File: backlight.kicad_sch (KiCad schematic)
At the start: 32 parts

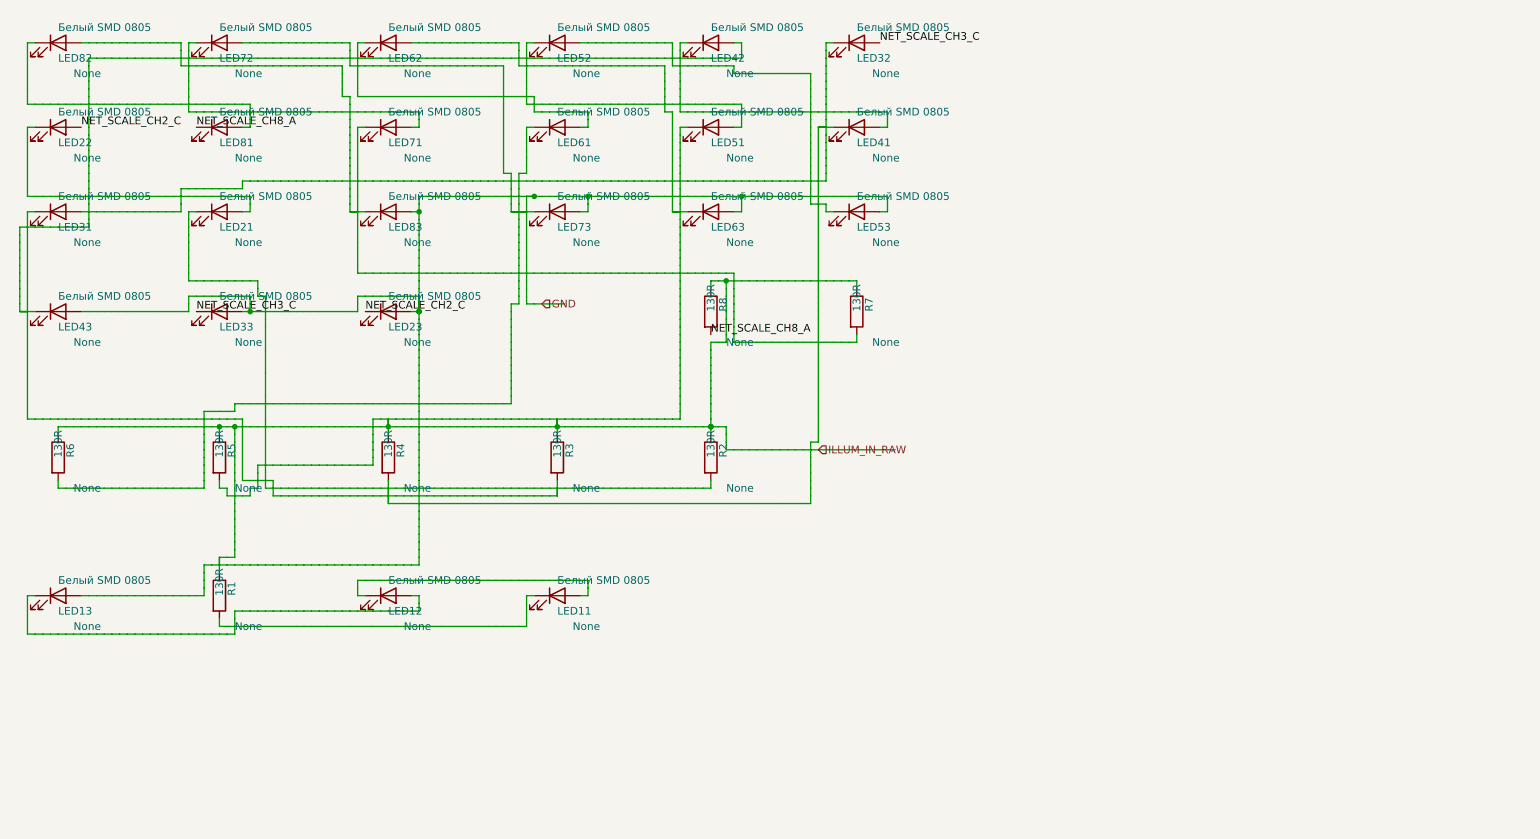
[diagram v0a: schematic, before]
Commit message: рефакторинг проекта и начала прогона тестов
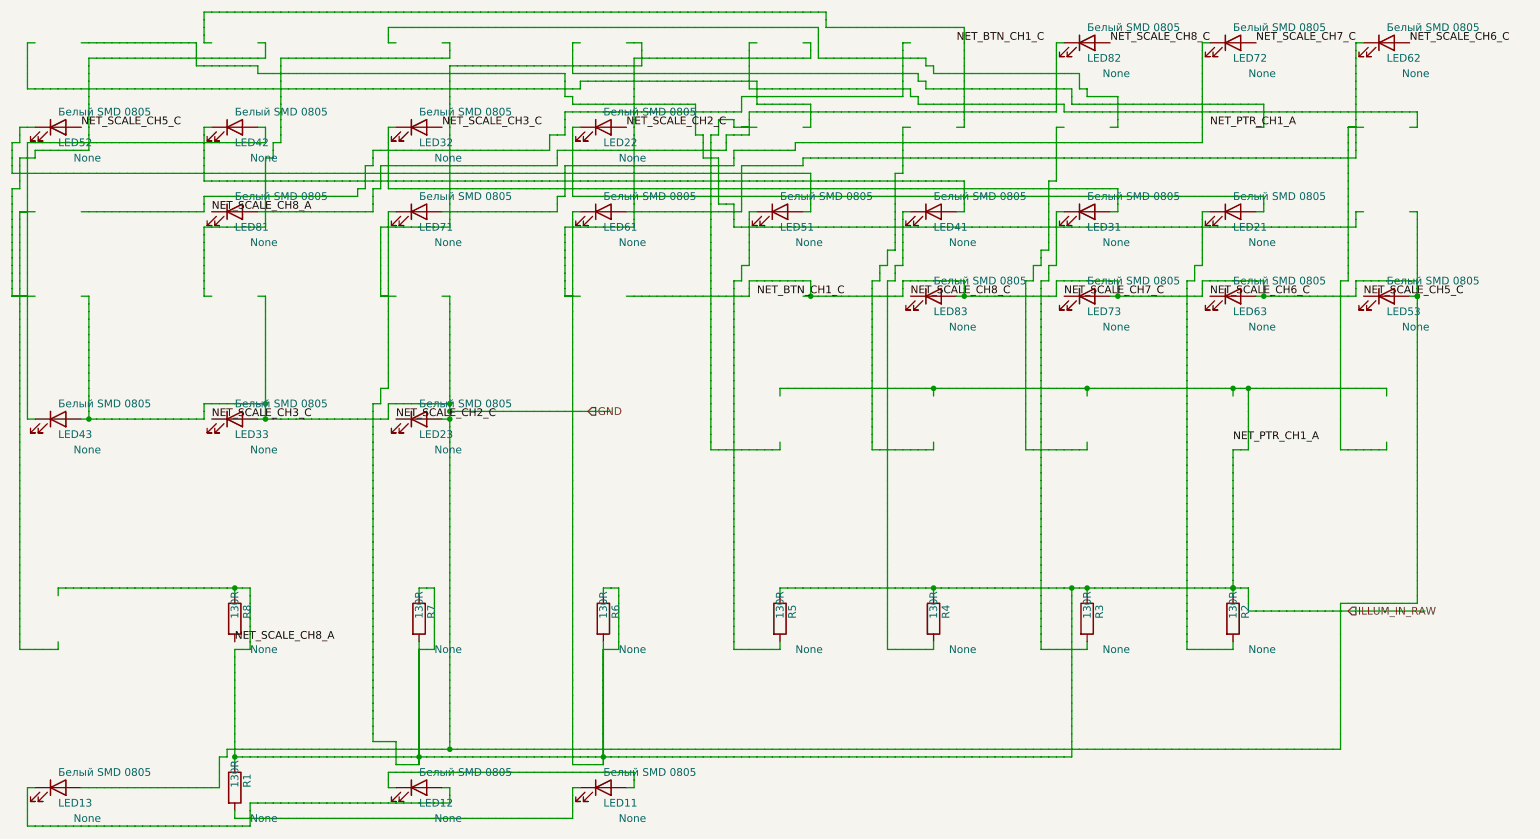
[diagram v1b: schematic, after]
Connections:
- net GND: no longer LED52.2 (A), LED53.1 (K), LED62.2 (A), LED63.1 (K), LED72.2 (A), LED73.1 (K), LED82.2 (A), LED83.1 (K)
- new net NET_SCALE_CH5_C: LED52.2 (A), LED53.1 (K)
- new net NET_SCALE_CH6_C: LED62.2 (A), LED63.1 (K)
- new net NET_SCALE_CH7_C: LED72.2 (A), LED73.1 (K)
- new net NET_SCALE_CH8_C: LED82.2 (A), LED83.1 (K)
